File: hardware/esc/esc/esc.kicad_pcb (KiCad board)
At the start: 4 copper layers, 28.3 x 28.3 mm, 171 parts, among them J1 JST SH 1.0mm, Q1 Q_NMOS, Q10 Q_NMOS, Q11 Q_NMOS, Q12 Q_NMOS, Q13 Q_NMOS, Q14 Q_NMOS, Q15 Q_NMOS, Q16 Q_NMOS, Q17 Q_NMOS, Q18 Q_NMOS, Q19 Q_NMOS, Q2 Q_NMOS, Q20 Q_NMOS, Q21 Q_NMOS, Q22 Q_NMOS, Q23 Q_NMOS, Q24 Q_NMOS, Q3 Q_NMOS, Q4 Q_NMOS, Q5 Q_NMOS, Q6 Q_NMOS, Q7 Q_NMOS, Q8 Q_NMOS, Q9 Q_NMOS, U1 NSG2065Q, U10 TLV76733DRVR, U11 LMR51420YDDCR, U2 AT32F421G8U7, U3 INA180B2, U4 AT32F421G8U7, U5 NSG2065Q, U6 AT32F421G8U7, U7 NSG2065Q, U8 AT32F421G8U7, U9 NSG2065Q

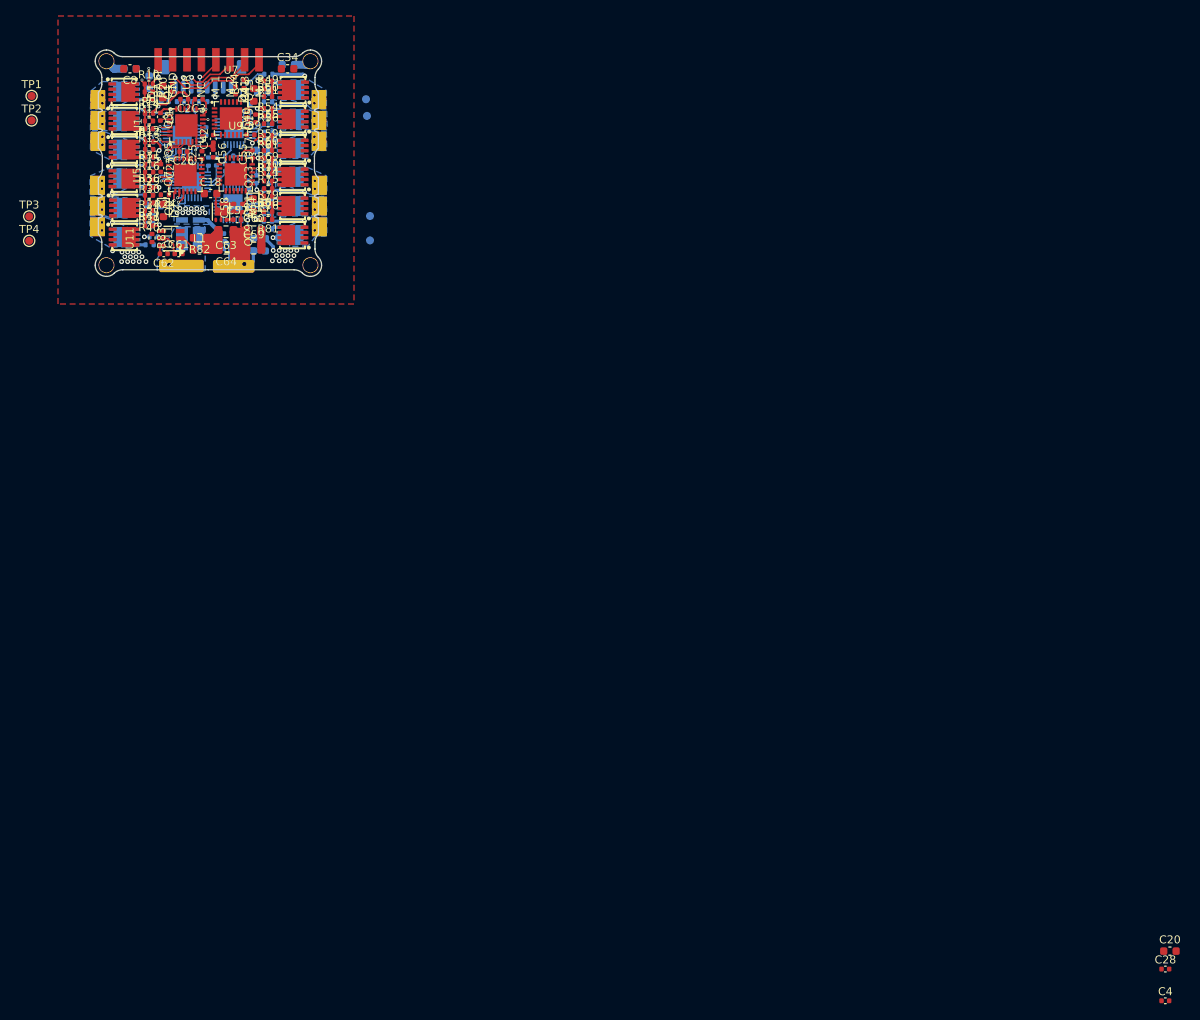
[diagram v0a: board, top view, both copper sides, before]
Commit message: Sync for windows
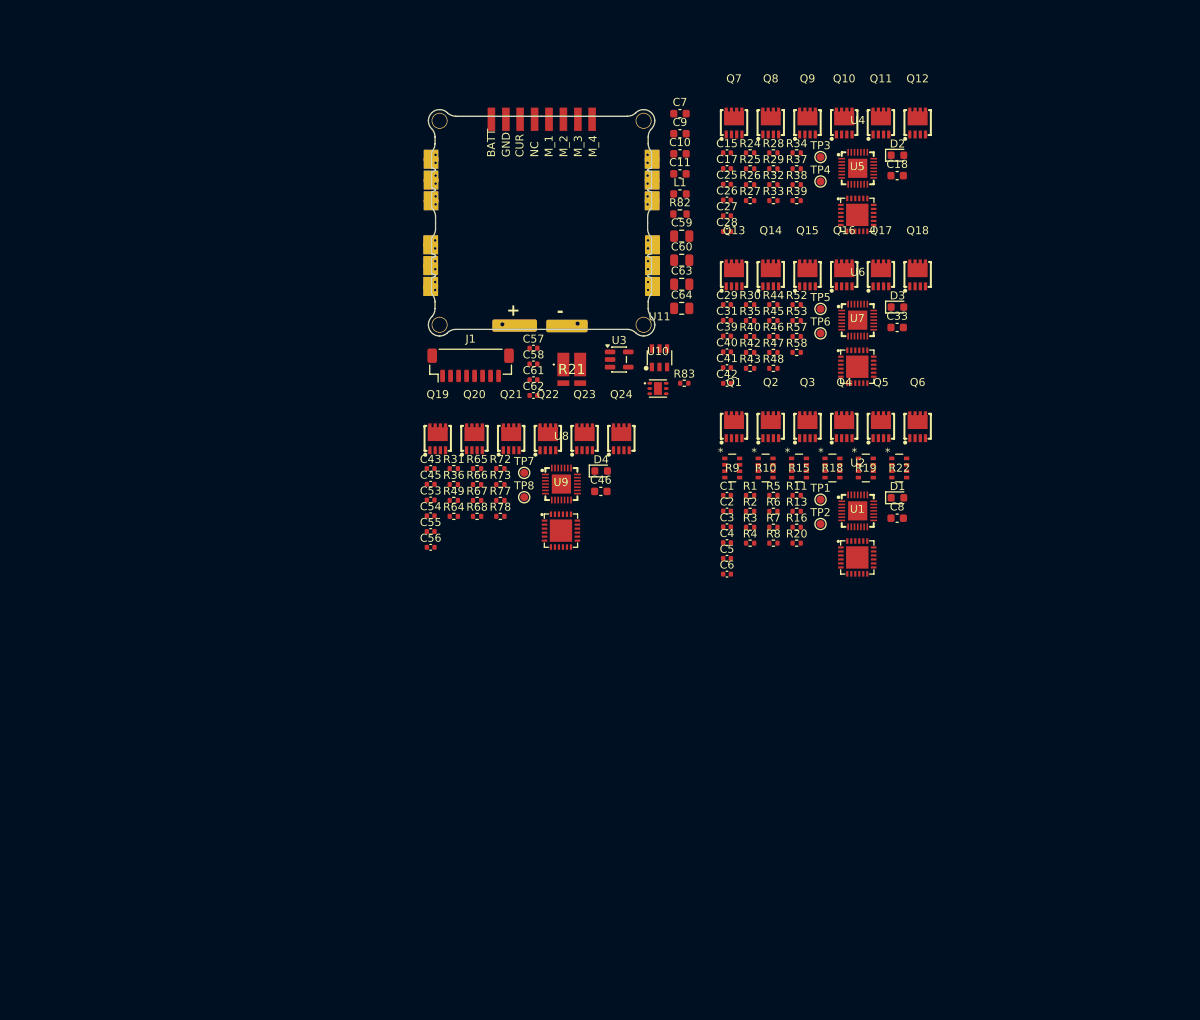
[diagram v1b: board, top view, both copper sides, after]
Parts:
- removed C19, C20, C32, C34, C47, C48: 10uF, Capacitor_SMD:C_0603_1608Metric
- removed R12, R14, R17, R41, R51, R54, R56, R59, R61, R69, R71, R74, R76, R79, R81: 10k, Resistor_SMD:R_0402_1005Metric
- removed R50, R55, R60, R70, R75, R80: 1k, Resistor_SMD:R_0402_1005Metric
- added C11: 22uF, Capacitor_SMD:C_0603_1608Metric, F.Cu at (88.7, 30.7)
- added C7: 22uF, Capacitor_SMD:C_0603_1608Metric, F.Cu at (88.7, 23.2)
- added R18: ~, R_Pack4:RES_4D03_0603_3P2X1P6_ROH, F.Cu at (107.8, 67.5)
- added R19: ~, R_Pack4:RES_4D03_0603_3P2X1P6_ROH, F.Cu at (112.0, 67.5)
- added R22: ~, R_Pack4:RES_4D03_0603_3P2X1P6_ROH, F.Cu at (116.2, 67.5)
- C10, C9: value 10uF -> 22uF; moved to F.Cu
- C15, C17, C29, C31, C43, C45, C5, C53, C54, C6, J1, Q10, Q12, Q14, Q16, Q18, Q2, Q20, Q22, Q24, Q4, Q6, Q8, R1, R2, R21, R25, R26, R27, R28, R3, R32, R33, R37, R38, R4, R42, R43, R45, R46, R47, R48, R5, R52, R53, R57, R58, R6, R65, R66, R67, R68, R7, R72, R73, R77, R78, R8, TP5, TP6, TP7, TP8, U2, U3, U4, U6, U8: moved to F.Cu
- C18, C8: value 10uF -> 4.7uF
- C33, C46: value 10uF -> 4.7uF; moved to F.Cu
- R10, R15, R9: value 10k -> ~; footprint Resistor_SMD:R_0402_1005Metric -> R_Pack4:RES_4D03_0603_3P2X1P6_ROH
- R29, R31, R34, R36, R39, R49: value 10k -> 1k
- moved C8 111.1 mm to (115.9, 73.8), turned to 0 degrees
- moved TP1 110.8 mm to (106.3, 71.5)
- moved TP2 110.8 mm to (106.3, 74.5)
- moved C28 107.2 mm to (94.6, 37.9)
- moved Q6 105.0 mm to (118.5, 62.3), turned to 0 degrees
- moved D1 104.9 mm to (115.9, 71.2), turned to 0 degrees
- moved Q5 100.7 mm to (113.9, 62.3), turned to 0 degrees
- moved Q12 100.2 mm to (118.5, 24.3), turned to 0 degrees
- moved U1 99.7 mm to (110.9, 78.7), turned to 0 degrees
- moved TP3 99.2 mm to (106.3, 28.6)
- moved TP4 99.2 mm to (106.3, 31.7)
- moved Q4 97.8 mm to (109.3, 62.3), turned to 0 degrees
- moved U2 96.6 mm to (111.0, 72.9), turned to 0 degrees
- moved R20 96.6 mm to (103.3, 76.9), turned to 0 degrees
- moved Q11 95.6 mm to (113.9, 24.3), turned to 0 degrees
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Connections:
- R10 pad 1: /ESC1/BEMF_A -> /ESC1/BEMF_COM
- R10 pad 2: /ESC1/FloatA -> /ESC1/BEMF_B
- R29 pad 1: /ESC2/BEMF_COM -> GND
- R30 pad 2: /ESC2/BEMF_A -> /ESC3/BEMF_A
- R31 pad 1: /ESC2/BEMF_A -> GND
- R31 pad 2: /ESC2/FloatA -> /ESC4/BEMF_A
- R34 pad 1: /ESC2/BEMF_COM -> GND
- R35 pad 2: /ESC2/BEMF_B -> /ESC3/BEMF_B
- R36 pad 1: /ESC2/BEMF_B -> GND
- R36 pad 2: /ESC2/FloatB -> /ESC4/BEMF_B
- R39 pad 1: /ESC2/BEMF_COM -> GND
- R40 pad 2: /ESC2/BEMF_C -> /ESC3/BEMF_C
- R49 pad 1: /ESC3/BEMF_COM -> GND
- R49 pad 2: /ESC3/BEMF_A -> /ESC4/BEMF_C
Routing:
- net GND: track 57.8 -> 0.00 mm, vias 1 -> 0
- net /ESC1/BEMF_COM: track 25.5 -> 0.00 mm, vias 2 -> 0
- net /ESC1/FloatC: track 20.4 -> 0.00 mm, vias 2 -> 0
- net /CURR_SENSE: track 20.4 -> 0.00 mm, vias 2 -> 0
- net /ESC1/FloatA: track 15.9 -> 0.00 mm, vias 2 -> 0
- net +8V: track 15.6 -> 0.00 mm
- net /ESC1/BEMF_B: track 15.6 -> 0.00 mm, vias 2 -> 0
- net /ESC1/FloatB: track 15.2 -> 0.00 mm, vias 1 -> 0
- net /ESC1/BEMF_A: track 14.5 -> 0.00 mm, vias 2 -> 0
- net /dshot_4: track 13.9 -> 0.00 mm, vias 1 -> 0
- net +BATT: track 13.2 -> 0.00 mm, vias 37 -> 0
- net /ESC1/BEMF_C: track 11.3 -> 0.00 mm, vias 2 -> 0
- net +3.3V: track 11.1 -> 0.00 mm
- net /dshot_3: track 10.8 -> 0.00 mm, vias 1 -> 0
- net /ESC4/FloatA: track 10.8 -> 0.00 mm, vias 1 -> 0
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- removed copper zone on B.Cu, net +BATT
- removed copper zone on F.Cu, net +BATT
- removed copper zone on In2.Cu, net +BATT
- removed copper zone on B.Cu, net /ESC1/FloatA
- removed copper zone on B.Cu, net /ESC1/FloatB
- removed copper zone on B.Cu, net /ESC1/FloatC
- removed copper zone on B.Cu, net /ESC2/FloatA
- removed copper zone on B.Cu, net /ESC2/FloatB
- removed copper zone on B.Cu, net /ESC2/FloatC
- removed copper zone on B.Cu, net /ESC3/FloatA
- removed copper zone on B.Cu, net /ESC3/FloatB
- removed copper zone on B.Cu, net /ESC3/FloatC
- removed copper zone on B.Cu, net /ESC4/FloatA
- removed copper zone on B.Cu, net /ESC4/FloatB
- removed copper zone on B.Cu, net /ESC4/FloatC
- removed copper zone on B.Cu, net /VBAT
- removed copper zone on B.Cu, net GND
- removed copper zone on In1.Cu, net GND
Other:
- outline, holes or cut-outs redrawn
